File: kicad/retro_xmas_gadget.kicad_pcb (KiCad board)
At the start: 2 copper layers, 66 x 86.4 mm, 18 parts, among them J1 USB_C_Receptacle_USB2.0_16P, J2 SD_Card_Receptacle, J3 AudioJack3_SwitchTR, Q1 UMH3N, SW3 SW_SPDT, U1 CP2102N-Axx-xQFN28, U2 ESP32-S3-WROOM-1

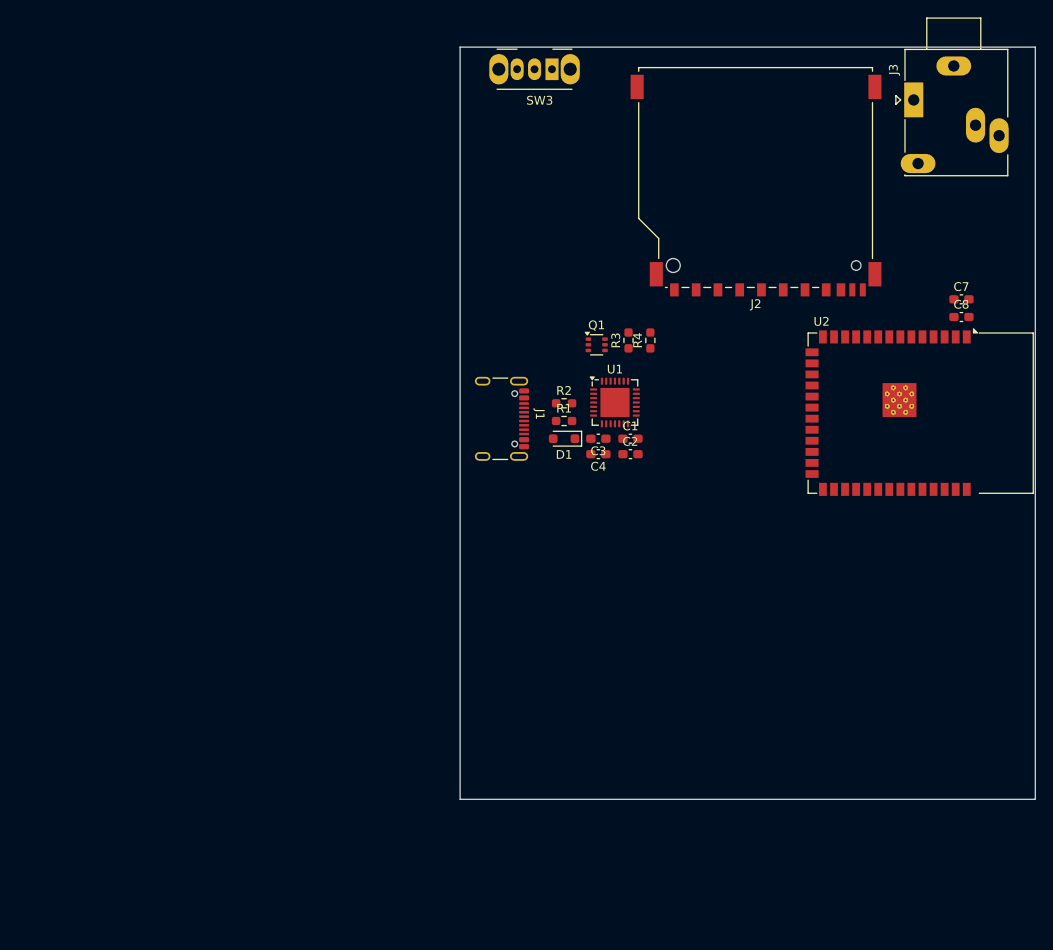
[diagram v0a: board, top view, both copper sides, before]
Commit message: complete most of design
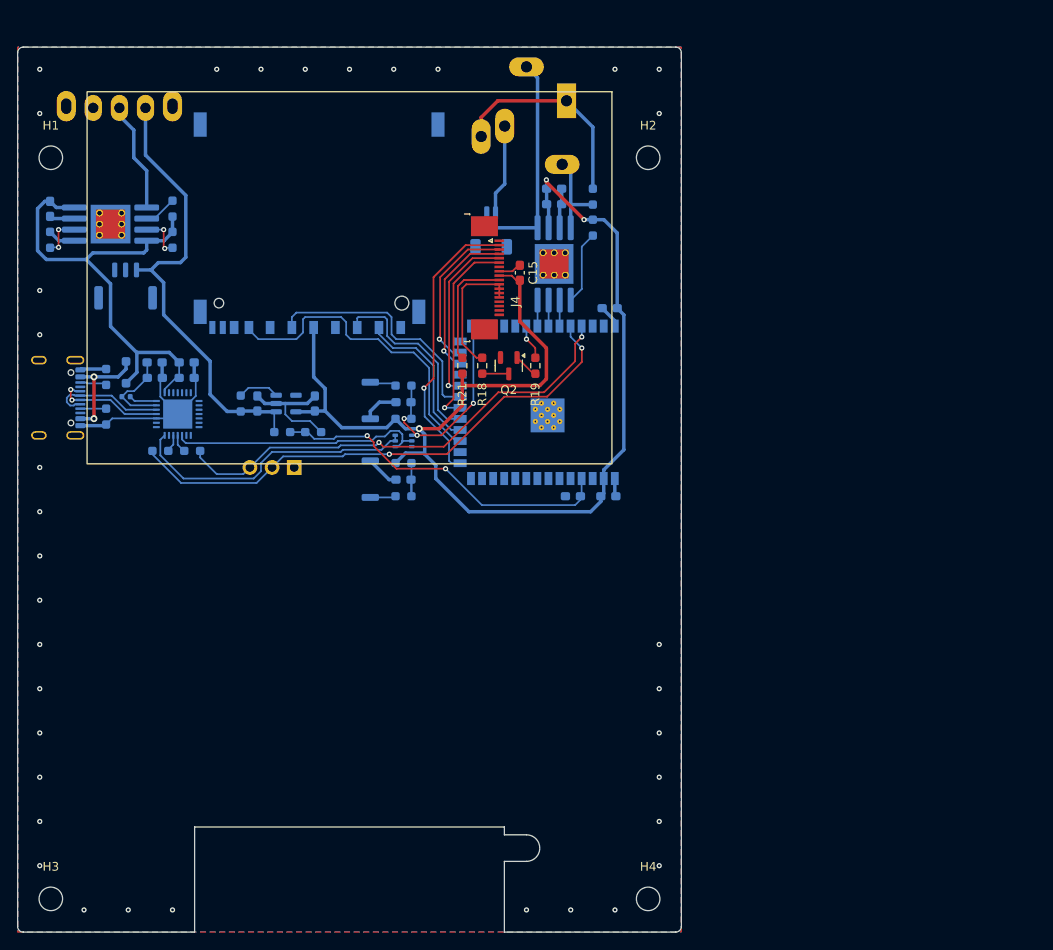
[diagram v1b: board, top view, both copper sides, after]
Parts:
- added C10: 100nf, Capacitor_SMD:C_0603_1608Metric_Pad1.08x0.95mm_HandSolder, B.Cu at (87.0, 68.8)
- added C11: 100nf, Capacitor_SMD:C_0603_1608Metric_Pad1.08x0.95mm_HandSolder, B.Cu at (89.2, 102.4)
- added C12: 10uf, Capacitor_SMD:C_0603_1608Metric_Pad1.08x0.95mm_HandSolder, B.Cu at (52.9, 91.7)
- added C13: 10uf, Capacitor_SMD:C_0603_1608Metric_Pad1.08x0.95mm_HandSolder, B.Cu at (59.5, 91.7)
- added C14: 100nf, Capacitor_SMD:C_0603_1608Metric_Pad1.08x0.95mm_HandSolder, B.Cu at (29.1, 69.4)
- added C15: 100nf, Capacitor_SMD:C_0603_1608Metric_Pad1.08x0.95mm_HandSolder, F.Cu at (83.1, 76.7)
- added C5: 100nf, Capacitor_SMD:C_0603_1608Metric_Pad1.08x0.95mm_HandSolder, B.Cu at (69.7, 100.5)
- added C6: 100nf, Capacitor_SMD:C_0603_1608Metric_Pad1.08x0.95mm_HandSolder, B.Cu at (69.7, 91.6)
- added C9: 10uf, Capacitor_SMD:C_0603_1608Metric_Pad1.08x0.95mm_HandSolder, B.Cu at (87.0, 67.1)
- added H1: MountingHole, MountingHole:MountingHole_2.7mm_M2.5, F.Cu at (29.2, 63.5)
- added H2: MountingHole, MountingHole:MountingHole_2.7mm_M2.5, F.Cu at (97.8, 63.5)
- added H3: MountingHole, MountingHole:MountingHole_2.7mm_M2.5, F.Cu at (29.2, 148.6)
- added H4: MountingHole, MountingHole:MountingHole_2.7mm_M2.5, F.Cu at (97.8, 148.6)
- added J4: Conn_01x18, Connector_FFC-FPC:TE_1-1734839-8_1x18-1MP_P0.5mm_Horizontal, F.Cu at (79.3, 77.3)
- added J5: Conn_01x02, Connector_JST:JST_SH_SM02B-SRSS-TB_1x02-1MP_P1.00mm_Horizontal, B.Cu at (79.8, 71.8)
- added J6: Conn_01x03, Connector_JST:JST_GH_SM03B-GHS-TB_1x03-1MP_P1.25mm_Horizontal, B.Cu at (37.8, 78.2)
- added J7: Conn_01x03, Connector_PinHeader_2.54mm:PinHeader_1x03_P2.54mm_Vertical, B.Cu at (57.1, 99.1)
- added Q2: SS8050, Package_TO_SOT_SMD:SOT-23, F.Cu at (81.8, 87.4)
- added R10: 470, Resistor_SMD:R_0603_1608Metric_Pad0.98x0.95mm_HandSolder, B.Cu at (91.4, 68.0)
- added R11: 100K, Resistor_SMD:R_0603_1608Metric_Pad0.98x0.95mm_HandSolder, B.Cu at (55.8, 95.0)
- added R12: 100K, Resistor_SMD:R_0603_1608Metric_Pad0.98x0.95mm_HandSolder, B.Cu at (59.3, 95.0)
- added R13: 10k, Resistor_SMD:R_0603_1608Metric_Pad0.98x0.95mm_HandSolder, B.Cu at (51.0, 91.7)
- added R14: 2K, Resistor_SMD:R_0603_1608Metric_Pad0.98x0.95mm_HandSolder, B.Cu at (29.1, 72.9)
- added R15: 5.1k, Resistor_SMD:R_0603_1608Metric_Pad0.98x0.95mm_HandSolder, B.Cu at (43.2, 69.3)
- added R16: 1k, Resistor_SMD:R_0603_1608Metric_Pad0.98x0.95mm_HandSolder, B.Cu at (43.2, 72.9)
- added R17: 0, Capacitor_SMD:C_0402_1005Metric, B.Cu at (37.8, 90.9)
- added R18: 0, Resistor_SMD:R_0603_1608Metric_Pad0.98x0.95mm_HandSolder, F.Cu at (78.7, 87.4)
- added R19: 1K, Resistor_SMD:R_0603_1608Metric_Pad0.98x0.95mm_HandSolder, F.Cu at (84.8, 87.4)
- added R21: 10R, Resistor_SMD:R_0603_1608Metric_Pad0.98x0.95mm_HandSolder, F.Cu at (76.5, 87.4)
- added R5: 220, Resistor_SMD:R_0603_1608Metric_Pad0.98x0.95mm_HandSolder, B.Cu at (69.7, 102.4)
- added R6: 220, Resistor_SMD:R_0603_1608Metric_Pad0.98x0.95mm_HandSolder, B.Cu at (69.7, 89.7)
- added R7: 10k, Resistor_SMD:R_0603_1608Metric_Pad0.98x0.95mm_HandSolder, B.Cu at (69.7, 98.6)
- added R8: 10k, Resistor_SMD:R_0603_1608Metric_Pad0.98x0.95mm_HandSolder, B.Cu at (69.7, 93.5)
- added R9: 10k, Resistor_SMD:R_0603_1608Metric_Pad0.98x0.95mm_HandSolder, B.Cu at (91.4, 71.5)
- added SW1: RESET, Button_Switch_SMD:SW_Push_SPST_NO_Alps_SKRK, B.Cu at (65.9, 100.4)
- added SW2: BOOT, Button_Switch_SMD:SW_Push_SPST_NO_Alps_SKRK, B.Cu at (65.9, 91.4)
- added U3: ~, Package_SO:SOP-8-1EP_4.57x4.57mm_P1.27mm_EP4.57x4.45mm_ThermalVias, B.Cu at (87.0, 75.7)
- added U4: XC6210B332MR, Package_TO_SOT_SMD:SOT-23-5, B.Cu at (56.2, 91.7)
- added U5: TP4056, Package_SO:SOP-8-1EP_4.57x4.57mm_P1.27mm_EP4.57x4.45mm_ThermalVias, B.Cu at (36.1, 71.1)
- C1, C2, C3, C4, C7, C8, D1, J1, J2, J3, Q1, R1, R2, R3, R4, U1, U2: moved to B.Cu
- SW3: value SW_SPDT -> KH-SS12F23-G6; moved to B.Cu
- moved R3 55.2 mm to (41.8, 97.2), turned to 180 degrees
- moved R4 54.1 mm to (45.4, 97.2), turned to 0 degrees
- moved SW3 52.9 mm to (34.1, 57.8), turned to 0 degrees
- moved R1 52.8 mm to (35.6, 88.7), turned to 90 degrees
- moved R2 52.6 mm to (35.6, 93.2), turned to -90 degrees
- moved C4 52.0 mm to (41.1, 87.0), turned to 0 degrees
- moved C2 52.0 mm to (44.8, 87.0)
- moved C1 51.4 mm to (44.8, 88.8)
- moved C3 51.4 mm to (41.1, 88.8), turned to 0 degrees
- moved J1 51.0 mm to (28.9, 91.1), turned to 90 degrees
- moved D1 50.9 mm to (37.8, 88.1), turned to 90 degrees
- moved J2 50.4 mm to (60.0, 71.0), turned to 0 degrees
- moved U1 50.2 mm to (43.8, 92.9)
- moved C8 45.5 mm to (93.2, 102.4)
- moved U2 40.4 mm to (88.7, 91.6), turned to 90 degrees
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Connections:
- net /IO10 renamed /SD_CD
- net /IO11 renamed /SD_CMD
- net /IO13 renamed /SD_CLK
- net /IO9 renamed /SD_DAT
- J3 pad R: unconnected-(J3-PadR) -> /HJ+
- J3 pad RN: unconnected-(J3-PadRN) -> /SPK+
- J3 pad S: unconnected-(J3-PadS) -> /AUDIO-
- J3 pad T: unconnected-(J3-PadT) -> /HJ+
- J3 pad TN: unconnected-(J3-PadTN) -> /AUDIO+
- SW3 pad 2: unconnected-(SW3-B-Pad2) -> /VBAT
- SW3 pad 3: unconnected-(SW3-C-Pad3) -> /VBAT_ON
- U1 pad 7: Net-(U1-VDD) -> Net-(U1-VREGIN)
- U2 pad 15: /IO3 -> /TFT_RST
- U2 pad 20: /IO12 -> /TFT_SDI
- U2 pad 22: /IO14 -> /TFT_CS
- U2 pad 24: /IO47 -> /TFT_DC
- U2 pad 25: /IO48 -> /TFT_SCL
- U2 pad 32: /IO39 -> /TFT_LED
- U2 pad 33: /IO40 -> /AMP_DATA
- U2 pad 34: /IO41 -> /AMP_BCLK
- U2 pad 35: /IO42 -> /AMP_LRCLK
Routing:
- net VCC: track 0.00 -> 140.7 mm, vias 0 -> 3
- net GND: track 0.00 -> 68.9 mm, vias 0 -> 35
- net /RXD: track 0.00 -> 61.5 mm, vias 0 -> 2
- net VBUS: track 0.00 -> 56.2 mm
- net /TXD: track 0.00 -> 54.7 mm, vias 0 -> 2
- net /VBAT_ON: track 0.00 -> 53.3 mm
- net /IO4: track 0.00 -> 39.8 mm, vias 0 -> 2
- net /SD_DAT: track 0.00 -> 36.8 mm
- net DTR: track 0.00 -> 33.6 mm
- net /TFT_RST: track 0.00 -> 33.2 mm, vias 0 -> 1
- net RTS: track 0.00 -> 29.7 mm
- net /SD_CLK: track 0.00 -> 28.1 mm
- net /AUDIO-: track 0.00 -> 26.0 mm
- net /IO0: track 0.00 -> 24.8 mm, vias 0 -> 3
- net /HJ+: track 0.00 -> 24.1 mm
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- added copper zone on B.Cu, net GND
- added copper zone on F.Cu, net GND
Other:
- board size 66 x 86.4 mm -> 76.2 x 101.6 mm
